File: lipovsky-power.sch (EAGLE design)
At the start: 99 parts, among them Q11 NMOS40V_10A, Q12 NMOS40V_10A, Q14 NMOS40V_10A, Q15 NMOS40V_10A, Q16 NMOS40V_10A, Q18 NMOS40V_10A, Q2 2NMOS30V_0.1A, Q21 PMOS30V_11A, Q22 PMOS30V_11A, Q23 NMOS40V_10A, Q24 NMOS40V_10A, Q25 PMOS30V_11A, Q26 PMOS30V_11A, Q27 NMOS40V_10A, Q28 NMOS40V_10A, Q3 2PMOS50V_0.17A, Q31 PMOS30V_11A, Q32 PMOS30V_11A, Q33 PMOS30V_11A, Q34 PMOS30V_11A, Q35 PMOS30V_11A, Q36 PMOS30V_11A, Q37 PMOS30V_11A, Q38 PMOS30V_11A, Q4 2PMOS50V_0.17A, Q41 PMOS30V_11A, Q42 PMOS30V_11A, Q43 PMOS30V_11A, Q44 PMOS30V_11A, Q45 PMOS30V_11A, Q46 PMOS30V_11A, Q47 PMOS30V_11A, Q48 PMOS30V_11A, Q5 2NMOS30V_0.1A, Q51 PMOS30V_11A, Q52 PMOS30V_11A, Q53 PMOS30V_11A, Q54 PMOS30V_11A, Q55 PMOS30V_11A, Q56 PMOS30V_11A, Q57 PMOS30V_11A, Q58 PMOS30V_11A, Q62 PMOS30V_11A, Q64 PMOS30V_11A, Q66 PMOS30V_11A, Q68 PMOS30V_11A, T1 TFORM_4_4311_4A4, U1 DG508BEN-T1-GE4, U2 DG508BEN-T1-GE4, U3 74HC595, U4 LTC3805-5IDD, U5 TC1240A, U6 AR30N60PPA-13

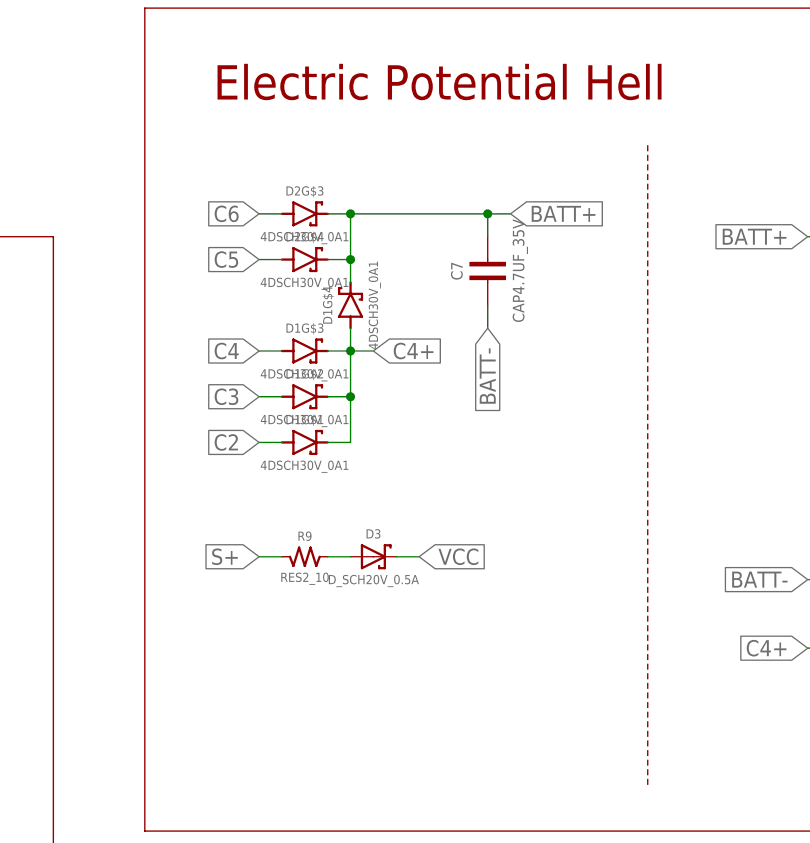
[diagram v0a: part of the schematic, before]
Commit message: organizing
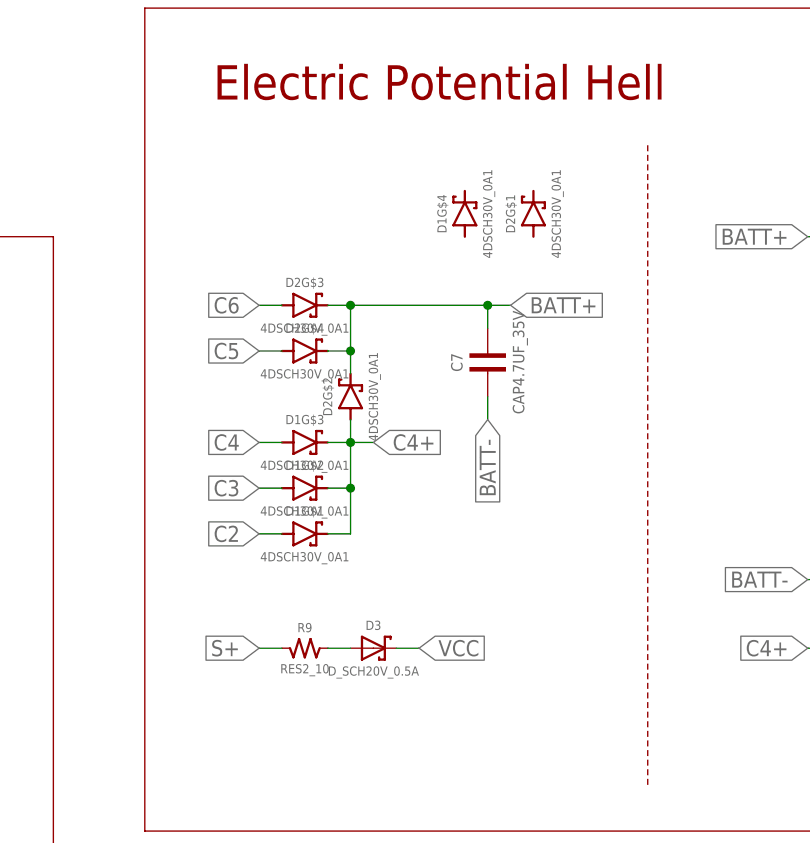
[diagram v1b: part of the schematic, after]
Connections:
- net BATT+: now also D2G$2.C; no longer D1G$4.C
- net C4+: now also D2G$2.A; no longer D1G$4.A
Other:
- moved on the sheet: C7, D1G$1, D1G$2, D1G$3, D1G$4, D2G$3, D2G$4, D3, R9
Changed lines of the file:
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@@
 <instance part="Q66" gate="G$1" x="-30.48" y="50.8" rot="MR90"/>
 <instance part="Q18" gate="G$1" x="-30.48" y="-53.34" rot="R270"/>
-<instance part="D1" gate="G$1" x="22.86" y="48.26"/>
-<instance part="D1" gate="G$2" x="22.86" y="53.34"/>
-<instance part="D1" gate="G$3" x="22.86" y="58.42"/>
-<instance part="D1" gate="G$4" x="27.94" y="63.5" rot="R90"/>
-<instance part="D2" gate="G$3" x="22.86" y="73.66"/>
+<instance part="D1" gate="G$1" x="22.86" y="38.1"/>
+<instance part="D1" gate="G$2" x="22.86" y="43.18"/>
+<instance part="D1" gate="G$3" x="22.86" y="48.26"/>
+<instance part="D1" gate="G$4" x="40.64" y="73.66" rot="R90"/>
+<instance part="D2" gate="G$3" x="22.86" y="63.5"/>
 <instance part="R1" gate="G$1" x="-76.2" y="-48.26" rot="R90"/>
 <instance part="R2" gate="G$1" x="-20.32" y="-48.26" rot="R90"/>
@@
 <instance part="Q24" gate="G$1" x="-86.36" y="-35.56" rot="R270"/>
 <instance part="RGS1" gate="G$1" x="86.36" y="25.4"/>
-<instance part="D2" gate="G$4" x="22.86" y="68.58"/>
+<instance part="D2" gate="G$4" x="22.86" y="58.42"/>
 <instance part="RGS-2" gate="G$1" x="86.36" y="33.02"/>
 <instance part="Q2" gate="G$2" x="99.06" y="25.4" rot="MR270"/>
@@
 <instance part="U4" gate="G$1" x="76.2" y="-55.88"/>
 <instance part="R8" gate="G$1" x="99.06" y="-58.42"/>
-<instance part="R9" gate="G$1" x="22.86" y="35.56"/>
-<instance part="D3" gate="G$1" x="30.48" y="35.56"/>
+<instance part="R9" gate="G$1" x="22.86" y="25.4"/>
+<instance part="D3" gate="G$1" x="30.48" y="25.4"/>
 <instance part="R10" gate="G$1" x="116.84" y="27.94" rot="R90"/>
 <instance part="C3" gate="G$1" x="43.18" y="-27.94" rot="R90"/>
-<instance part="C7" gate="G$1" x="43.18" y="66.04" rot="R90"/>
+<instance part="C7" gate="G$1" x="43.18" y="55.88" rot="R90"/>
 <instance part="C8" gate="G$1" x="261.62" y="76.2"/>
 <instance part="U6" gate="G$1" x="187.96" y="-43.18"/>
@@
 <instance part="Q5" gate="G$2" x="152.4" y="-68.58" rot="R90"/>
 <instance part="Q3" gate="G$2" x="132.08" y="22.86" rot="R270"/>
+<instance part="D2" gate="G$1" x="48.26" y="73.66" rot="R90"/>
+<instance part="D2" gate="G$2" x="27.94" y="53.34" rot="R90"/>
 </instances>
 <busses>
@@
 </segment>
 <segment>
-<wire x1="20.32" y1="48.26" x2="17.78" y2="48.26" width="0.1524" layer="91"/>
-<label x="17.78" y="48.26" size="1.778" layer="95" rot="R180" xref="yes"/>
+<wire x1="20.32" y1="38.1" x2="17.78" y2="38.1" width="0.1524" layer="91"/>
+<label x="17.78" y="38.1" size="1.778" layer="95" rot="R180" xref="yes"/>
 <pinref part="D1" gate="G$1" pin="A"/>
 </segment>
@@
 </segment>
 <segment>
-<wire x1="20.32" y1="53.34" x2="17.78" y2="53.34" width="0.1524" layer="91"/>
-<label x="17.78" y="53.34" size="1.778" layer="95" rot="R180" xref="yes"/>
+<wire x1="20.32" y1="43.18" x2="17.78" y2="43.18" width="0.1524" layer="91"/>
+<label x="17.78" y="43.18" size="1.778" layer="95" rot="R180" xref="yes"/>
 <pinref part="D1" gate="G$2" pin="A"/>
 </segment>
@@
 </segment>
 <segment>
-<wire x1="20.32" y1="58.42" x2="17.78" y2="58.42" width="0.1524" layer="91"/>
-<label x="17.78" y="58.42" size="1.778" layer="95" rot="R180" xref="yes"/>
+<wire x1="20.32" y1="48.26" x2="17.78" y2="48.26" width="0.1524" layer="91"/>
+<label x="17.78" y="48.26" size="1.778" layer="95" rot="R180" xref="yes"/>
 <pinref part="D1" gate="G$3" pin="A"/>
 </segment>
@@
 </segment>
 <segment>
-<label x="17.78" y="68.58" size="1.778" layer="95" rot="R180" xref="yes"/>
+<label x="17.78" y="58.42" size="1.778" layer="95" rot="R180" xref="yes"/>
 <pinref part="D2" gate="G$4" pin="A"/>
-<wire x1="17.78" y1="68.58" x2="20.32" y2="68.58" width="0.1524" layer="91"/>
+<wire x1="17.78" y1="58.42" x2="20.32" y2="58.42" width="0.1524" layer="91"/>
 </segment>
 <segment>
@@
 <segment>
 <pinref part="D2" gate="G$3" pin="A"/>
-<wire x1="20.32" y1="73.66" x2="17.78" y2="73.66" width="0.1524" layer="91"/>
-<label x="17.78" y="73.66" size="1.778" layer="95" rot="R180" xref="yes"/>
+<wire x1="20.32" y1="63.5" x2="17.78" y2="63.5" width="0.1524" layer="91"/>
+<label x="17.78" y="63.5" size="1.778" layer="95" rot="R180" xref="yes"/>
 </segment>
 </net>
@@
 </segment>
 <segment>
-<wire x1="20.32" y1="35.56" x2="17.78" y2="35.56" width="0.1524" layer="91"/>
-<label x="17.78" y="35.56" size="1.778" layer="95" rot="R180" xref="yes"/>
+<wire x1="20.32" y1="25.4" x2="17.78" y2="25.4" width="0.1524" layer="91"/>
+<label x="17.78" y="25.4" size="1.778" layer="95" rot="R180" xref="yes"/>
 <pinref part="R9" gate="G$1" pin="1"/>
 </segment>
@@
 <segment>
 <pinref part="C7" gate="G$1" pin="1"/>
-<wire x1="43.18" y1="63.5" x2="43.18" y2="60.96" width="0.1524" layer="91"/>
-<label x="43.18" y="60.96" size="1.778" layer="95" rot="R270" xref="yes"/>
+<wire x1="43.18" y1="53.34" x2="43.18" y2="50.8" width="0.1524" layer="91"/>
+<label x="43.18" y="50.8" size="1.778" layer="95" rot="R270" xref="yes"/>
 </segment>
 </net>
@@
 <net name="VCC" class="0">
 <segment>
-<label x="35.56" y="35.56" size="1.778" layer="95" xref="yes"/>
-<wire x1="33.02" y1="35.56" x2="35.56" y2="35.56" width="0.1524" layer="91"/>
+<label x="35.56" y="25.4" size="1.778" layer="95" xref="yes"/>
+<wire x1="33.02" y1="25.4" x2="35.56" y2="25.4" width="0.1524" layer="91"/>
 <pinref part="D3" gate="G$1" pin="C"/>
 </segment>
@@
 </segment>
 <segment>
-<pinref part="D1" gate="G$4" pin="C"/>
 <pinref part="D2" gate="G$4" pin="C"/>
 <pinref part="D2" gate="G$3" pin="C"/>
-<wire x1="27.94" y1="73.66" x2="25.4" y2="73.66" width="0.1524" layer="91"/>
-<junction x="27.94" y="73.66"/>
-<wire x1="27.94" y1="73.66" x2="43.18" y2="73.66" width="0.1524" layer="91"/>
-<wire x1="43.18" y1="73.66" x2="45.72" y2="73.66" width="0.1524" layer="91"/>
-<wire x1="27.94" y1="73.66" x2="27.94" y2="68.58" width="0.1524" layer="91"/>
-<wire x1="27.94" y1="68.58" x2="25.4" y2="68.58" width="0.1524" layer="91"/>
-<junction x="27.94" y="68.58"/>
-<wire x1="27.94" y1="68.58" x2="27.94" y2="66.04" width="0.1524" layer="91"/>
-<label x="45.72" y="73.66" size="1.778" layer="95" xref="yes"/>
+<wire x1="27.94" y1="63.5" x2="25.4" y2="63.5" width="0.1524" layer="91"/>
+<junction x="27.94" y="63.5"/>
+<wire x1="27.94" y1="63.5" x2="43.18" y2="63.5" width="0.1524" layer="91"/>
+<wire x1="43.18" y1="63.5" x2="45.72" y2="63.5" width="0.1524" layer="91"/>
+<wire x1="27.94" y1="63.5" x2="27.94" y2="58.42" width="0.1524" layer="91"/>
+<wire x1="27.94" y1="58.42" x2="25.4" y2="58.42" width="0.1524" layer="91"/>
+<label x="45.72" y="63.5" size="1.778" layer="95" xref="yes"/>
 <pinref part="C7" gate="G$1" pin="2"/>
-<wire x1="43.18" y1="73.66" x2="43.18" y2="71.12" width="0.1524" layer="91"/>
-<junction x="43.18" y="73.66"/>
+<wire x1="43.18" y1="63.5" x2="43.18" y2="60.96" width="0.1524" layer="91"/>
+<junction x="43.18" y="63.5"/>
+<pinref part="D2" gate="G$2" pin="C"/>
+<wire x1="27.94" y1="55.88" x2="27.94" y2="58.42" width="0.1524" layer="91"/>
+<junction x="27.94" y="58.42"/>
 </segment>
 <segment>
@@
 <segment>
 <pinref part="D1" gate="G$3" pin="C"/>
-<wire x1="25.4" y1="58.42" x2="27.94" y2="58.42" width="0.1524" layer="91"/>
-<wire x1="27.94" y1="58.42" x2="27.94" y2="53.34" width="0.1524" layer="91"/>
+<wire x1="25.4" y1="48.26" x2="27.94" y2="48.26" width="0.1524" layer="91"/>
+<wire x1="27.94" y1="48.26" x2="27.94" y2="43.18" width="0.1524" layer="91"/>
 <pinref part="D1" gate="G$2" pin="C"/>
-<wire x1="27.94" y1="53.34" x2="25.4" y2="53.34" width="0.1524" layer="91"/>
-<wire x1="27.94" y1="53.34" x2="27.94" y2="48.26" width="0.1524" layer="91"/>
-<junction x="27.94" y="53.34"/>
+<wire x1="27.94" y1="43.18" x2="25.4" y2="43.18" width="0.1524" layer="91"/>
+<wire x1="27.94" y1="43.18" x2="27.94" y2="38.1" width="0.1524" layer="91"/>
+<junction x="27.94" y="43.18"/>
 <pinref part="D1" gate="G$1" pin="C"/>
-<wire x1="27.94" y1="48.26" x2="25.4" y2="48.26" width="0.1524" layer="91"/>
-<pinref part="D1" gate="G$4" pin="A"/>
-<wire x1="27.94" y1="58.42" x2="27.94" y2="60.96" width="0.1524" layer="91"/>
-<junction x="27.94" y="58.42"/>
-<wire x1="27.94" y1="58.42" x2="30.48" y2="58.42" width="0.1524" layer="91"/>
-<label x="30.48" y="58.42" size="1.778" layer="95" xref="yes"/>
+<wire x1="27.94" y1="38.1" x2="25.4" y2="38.1" width="0.1524" layer="91"/>
+<junction x="27.94" y="48.26"/>
+<wire x1="27.94" y1="48.26" x2="30.48" y2="48.26" width="0.1524" layer="91"/>
+<label x="30.48" y="48.26" size="1.778" layer="95" xref="yes"/>
+<pinref part="D2" gate="G$2" pin="A"/>
+<wire x1="27.94" y1="50.8" x2="27.94" y2="48.26" width="0.1524" layer="91"/>
 </segment>
 <segment>
@@
 <pinref part="R9" gate="G$1" pin="2"/>
 <pinref part="D3" gate="G$1" pin="A"/>
-<wire x1="25.4" y1="35.56" x2="27.94" y2="35.56" width="0.1524" layer="91"/>
-</segment>
-</net>
+<wire x1="25.4" y1="25.4" x2="27.94" y2="25.4" width="0.1524" layer="91"/>
+</segment>
+</net>
